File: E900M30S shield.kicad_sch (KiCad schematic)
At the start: 5 parts, among them J1 Conn10, J2 Conn02, U1 E22-900M30S

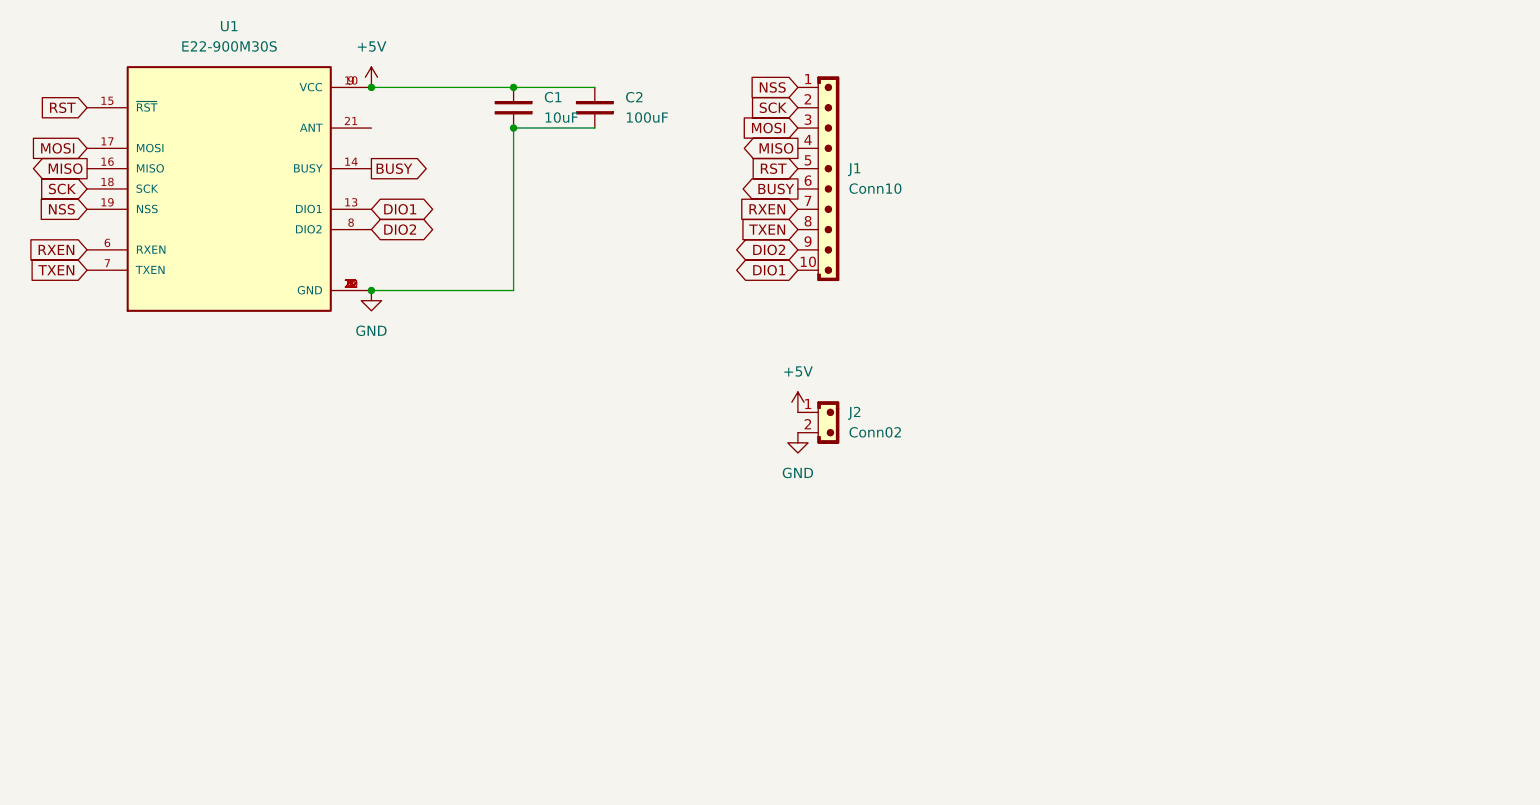
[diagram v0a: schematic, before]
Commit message: Final touches
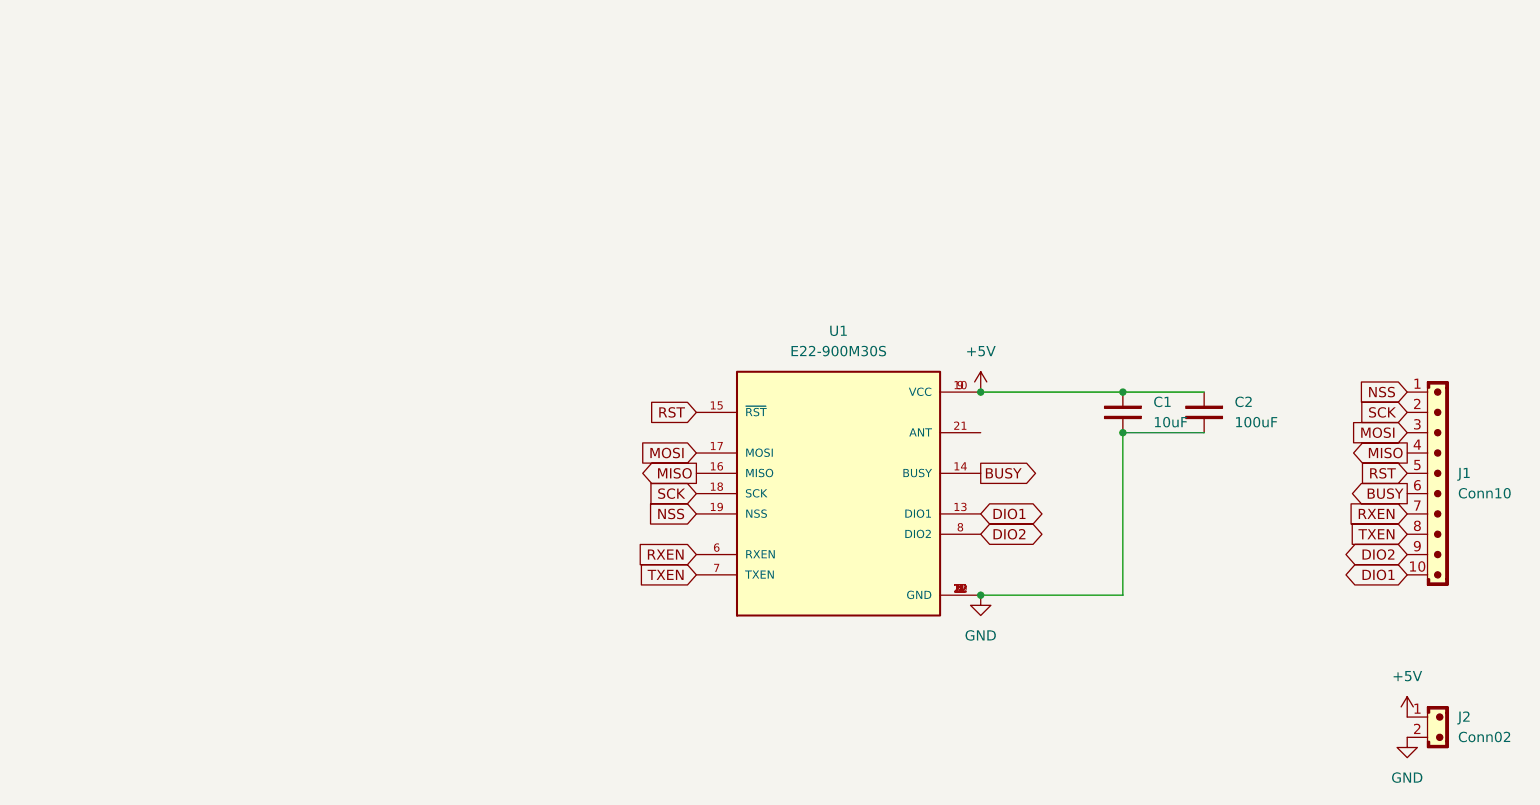
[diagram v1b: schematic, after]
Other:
- company: (none) -> Stefan Gofferje
- title: (none) -> Breakout board for eByte E22 SPI modules with CM4 footprint
- moved on the sheet: C1, C2, J1, J2, U1
